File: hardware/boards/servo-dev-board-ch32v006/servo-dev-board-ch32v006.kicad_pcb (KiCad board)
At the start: 4 copper layers, 50 x 50 mm, 81 parts, among them J1 BATT JST-PH, J2 BUS JST-ZH, J3 BUS JST-ZH, J4 SERVO JST-ZH, J5 ENC JST-ZH, J6 DBG JST-ZH, Q4 AO3400A, SW1 SW_Push, U1 HT75xx-1-SOT89, U3 DRV8837DSGR-JSM, U4 CH32V006F8U6

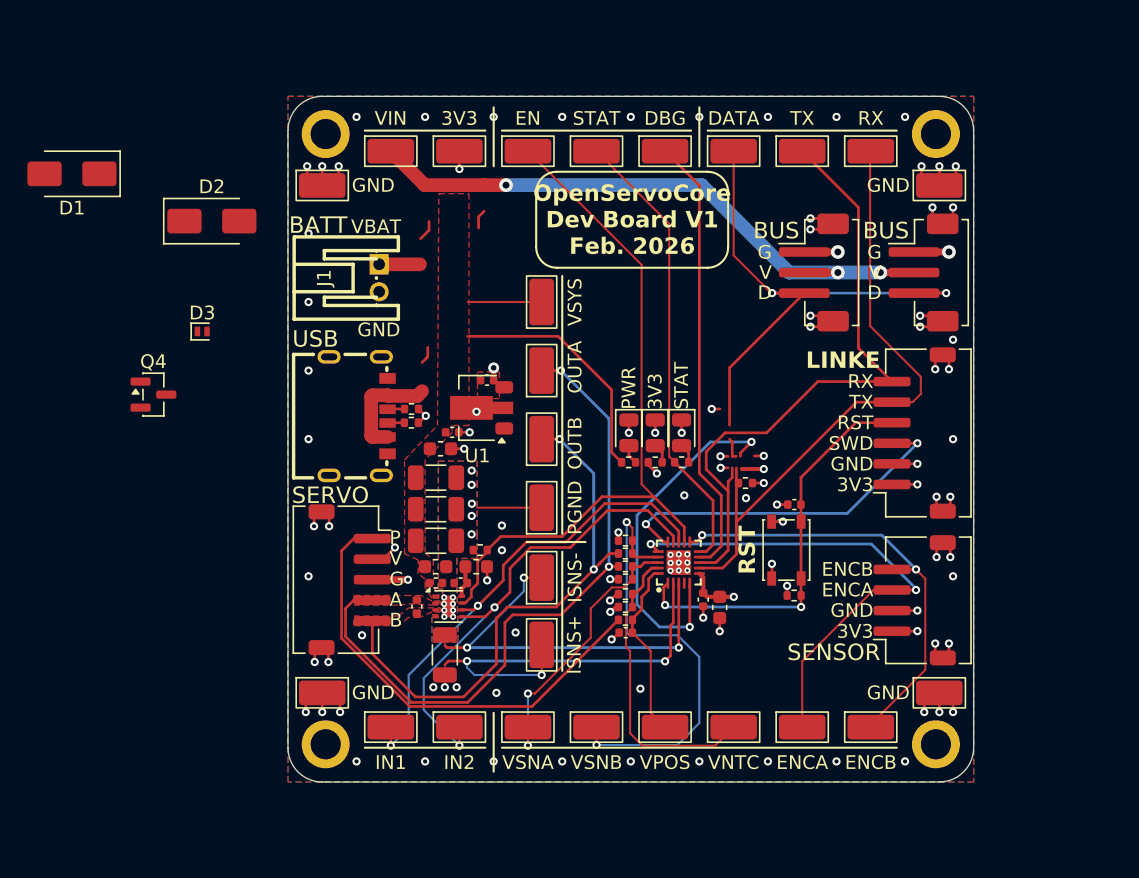
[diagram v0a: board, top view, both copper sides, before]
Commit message: completed rework
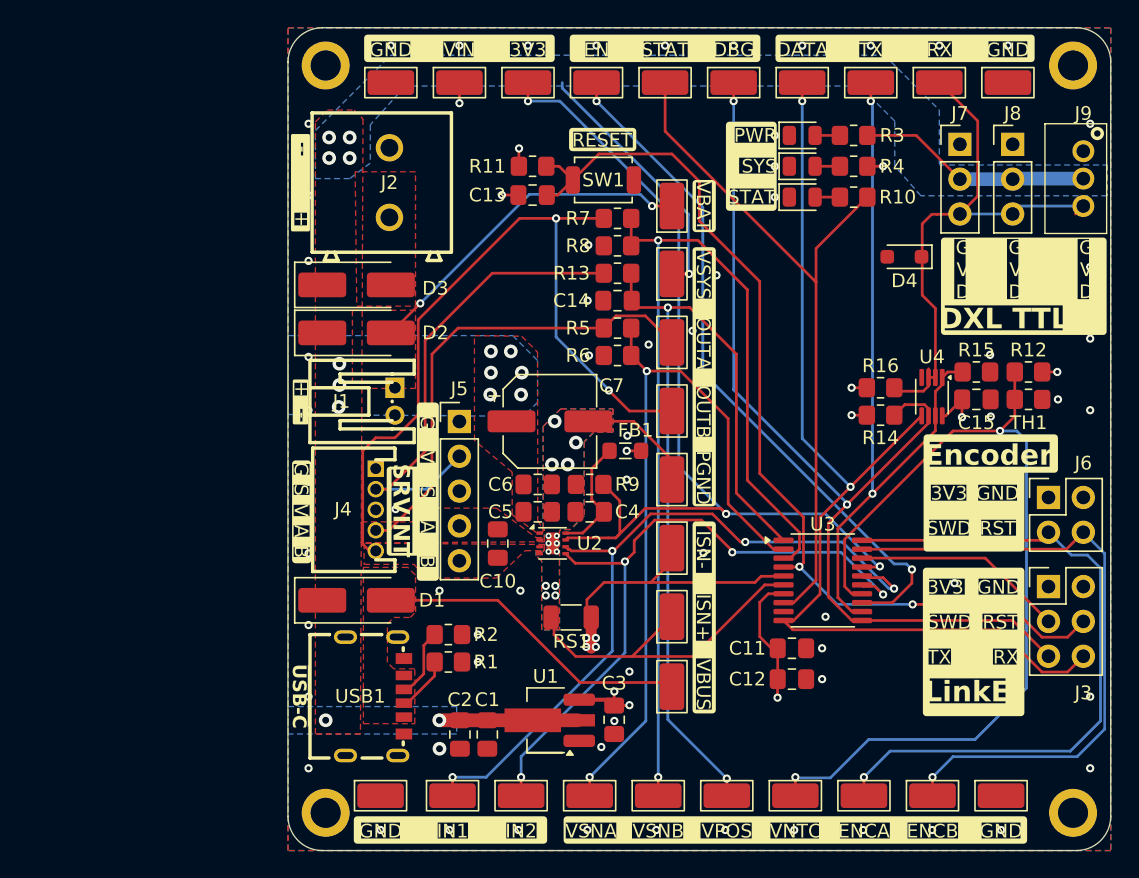
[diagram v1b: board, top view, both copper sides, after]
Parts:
- removed C8: 0.1µF, Capacitor_SMD:C_0402_1005Metric
- removed C9: 10µF, Capacitor_SMD:C_0603_1608Metric
- removed Q4: AO3400A, Package_TO_SOT_SMD:SOT-23
- removed R17: 20kΩ, Resistor_SMD:R_0402_1005Metric
- removed R18: 10kΩ, Resistor_SMD:R_0402_1005Metric
- added C4: 0.1µF, Capacitor_SMD:C_0805_2012Metric_Pad1.18x1.45mm_HandSolder, F.Cu at (152.0, 90.3)
- added D4: PESD5V0L1BA, Diode_SMD:D_SOD-323_HandSoldering, F.Cu at (174.9, 71.7)
- added J7: PIN-V, Connector_PinHeader_2.54mm:PinHeader_1x03_P2.54mm_Vertical, F.Cu at (179.0, 63.5)
- added J8: PIN-V, Connector_PinHeader_2.54mm:PinHeader_1x03_P2.54mm_Vertical, F.Cu at (182.8, 63.5)
- added J9: JST-PH-V, shared:CONN-TH_B3B-PH-K-S, F.Cu at (188.0, 66.0)
- added R1: 5.1kΩ, Resistor_SMD:R_0805_2012Metric_Pad1.20x1.40mm_HandSolder, F.Cu at (141.7, 101.2)
- added R2: 5.1kΩ, Resistor_SMD:R_0805_2012Metric_Pad1.20x1.40mm_HandSolder, F.Cu at (141.7, 99.2)
- added R3: 1.5kΩ, Resistor_SMD:R_0805_2012Metric_Pad1.20x1.40mm_HandSolder, F.Cu at (171.2, 62.9)
- added R5: 20kΩ, Resistor_SMD:R_0805_2012Metric_Pad1.20x1.40mm_HandSolder, F.Cu at (154.0, 76.9)
- added TP27: TestPoint_Probe, TestPoint:TestPoint_Keystone_5015_Micro_Mini, F.Cu at (158.0, 68.0)
- added TP28: TestPoint_Probe, TestPoint:TestPoint_Keystone_5015_Micro_Mini, F.Cu at (158.0, 103.0)
- added U2: DRV8212PDSGR, Package_SON:WSON-8-1EP_2x2mm_P0.5mm_EP0.9x1.6mm, F.Cu at (149.3, 92.6)
- C1: footprint Capacitor_SMD:C_0603_1608Metric -> Capacitor_SMD:C_0805_2012Metric_Pad1.18x1.45mm_HandSolder
- C10, C12: value 47µF -> 0.1µF; footprint Capacitor_SMD:C_1206_3216Metric -> Capacitor_SMD:C_0805_2012Metric_Pad1.18x1.45mm_HandSolder
- C11: value 47µF -> 10µF; footprint Capacitor_SMD:C_1206_3216Metric -> Capacitor_SMD:C_0805_2012Metric_Pad1.18x1.45mm_HandSolder
- C13, C15, C2, C3, C5: footprint Capacitor_SMD:C_0402_1005Metric -> Capacitor_SMD:C_0805_2012Metric_Pad1.18x1.45mm_HandSolder
- C14: value 10µF -> 0.1µF; footprint Capacitor_SMD:C_0603_1608Metric -> Capacitor_SMD:C_0805_2012Metric_Pad1.18x1.45mm_HandSolder
- C6: value 0.1µF -> 10µF; footprint Capacitor_SMD:C_0402_1005Metric -> Capacitor_SMD:C_0805_2012Metric_Pad1.18x1.45mm_HandSolder
- C7: value 0.1µF -> 100µF; footprint Capacitor_SMD:C_0402_1005Metric -> Capacitor_SMD:CP_Elec_6.3x5.4
- D1, D2: value SS34 -> SS54; footprint Diode_SMD:D_SMA -> Diode_SMD:D_SMA_Handsoldering
- D3: value ESD -> SS54; footprint Diode_SMD:D_SOD-882 -> Diode_SMD:D_SMA_Handsoldering
- FB1: footprint Inductor_SMD:L_0603_1608Metric -> Inductor_SMD:L_0805_2012Metric_Pad1.05x1.20mm_HandSolder
- J1: value BATT JST-PH -> JST-PH-H
- J2: value BUS JST-ZH -> TERM; footprint Connector_JST:JST_ZH_B3B-ZR-SM4-TF_1x03-1MP_P1.50mm_Vertical -> shared:CONN-TH_2P-P5.00_WJ500V-5.08-2P
- J3: value BUS JST-ZH -> PIN-V; footprint Connector_JST:JST_ZH_B3B-ZR-SM4-TF_1x03-1MP_P1.50mm_Vertical -> Connector_PinHeader_2.54mm:PinHeader_2x03_P2.54mm_Vertical
- J4: value SERVO JST-ZH -> JST-ZH-H; footprint Connector_JST:JST_ZH_S5B-ZR-SM4A-TF_1x05-1MP_P1.50mm_Horizontal -> shared:CONN-TH_S5B-ZR-LF-SN
- J5: value ENC JST-ZH -> PIN-V; footprint Connector_JST:JST_ZH_S4B-ZR-SM4A-TF_1x04-1MP_P1.50mm_Horizontal -> Connector_PinHeader_2.54mm:PinHeader_1x05_P2.54mm_Vertical
- J6: value DBG JST-ZH -> PIN-V; footprint Connector_JST:JST_ZH_S6B-ZR-SM4A-TF_1x06-1MP_P1.50mm_Horizontal -> Connector_PinHeader_2.54mm:PinHeader_2x02_P2.54mm_Vertical
- R10: value 5.1kΩ -> 1kΩ; footprint Resistor_SMD:R_0402_1005Metric -> Resistor_SMD:R_0805_2012Metric_Pad1.20x1.40mm_HandSolder
- R11: value 2.2kΩ -> 10kΩ; footprint Resistor_SMD:R_0402_1005Metric -> Resistor_SMD:R_0805_2012Metric_Pad1.20x1.40mm_HandSolder
- R12: value 330Ω -> 10kΩ; footprint Resistor_SMD:R_0402_1005Metric -> Resistor_SMD:R_0805_2012Metric_Pad1.20x1.40mm_HandSolder
- R13: value 1KΩ -> 4.7kΩ; footprint Resistor_SMD:R_0402_1005Metric -> Resistor_SMD:R_0805_2012Metric_Pad1.20x1.40mm_HandSolder
- R14, R16, R8: footprint Resistor_SMD:R_0402_1005Metric -> Resistor_SMD:R_0805_2012Metric_Pad1.20x1.40mm_HandSolder
- R15: value 20kΩ -> 10kΩ; footprint Resistor_SMD:R_0402_1005Metric -> Resistor_SMD:R_0805_2012Metric_Pad1.20x1.40mm_HandSolder
- R4: value 49.9Ω -> 470Ω; footprint Resistor_SMD:R_0402_1005Metric -> Resistor_SMD:R_0805_2012Metric_Pad1.20x1.40mm_HandSolder
- R6: value 4.7kΩ -> 10kΩ; footprint Resistor_SMD:R_0402_1005Metric -> Resistor_SMD:R_0805_2012Metric_Pad1.20x1.40mm_HandSolder
- R7: value 10kΩ -> 20kΩ; footprint Resistor_SMD:R_0402_1005Metric -> Resistor_SMD:R_0805_2012Metric_Pad1.20x1.40mm_HandSolder
- R9: value 5.1kΩ -> 10kΩ; footprint Resistor_SMD:R_0402_1005Metric -> Resistor_SMD:R_0805_2012Metric_Pad1.20x1.40mm_HandSolder
- RS1: value 0.1Ω 1% -> 100mΩ 1%
- SW1: footprint Button_Switch_SMD:SW_SPST_PTS810 -> Button_Switch_SMD:SW_SPST_TS-1088-xR020
- TH1: value NTC 10k -> 10kΩ 3950K; footprint Resistor_SMD:R_0402_1005Metric -> Resistor_SMD:R_0805_2012Metric_Pad1.20x1.40mm_HandSolder
- U1: value HT75xx-1-SOT89 -> HT7533-1; footprint Package_TO_SOT_SMD:SOT-89-3 -> Package_TO_SOT_SMD:SOT-89-3_Handsoldering
- U3: value DRV8837DSGR-JSM -> CH32V006F8P6; footprint Package_SON:WSON-8-1EP_2x2mm_P0.5mm_EP0.9x1.6mm -> Package_SO:TSSOP-20_4.4x6.5mm_P0.65mm
- U4: value CH32V006F8U6 -> 74LVC2G241; footprint shared:UQFN-20_L3.0-W3.0-P0.40-BL-EP1.7 -> Package_SO:VSSOP-8_2.3x2mm_P0.5mm
- USB1: value TYPE-C 6P(073) -> TYPE-C-H
- moved D1 37.4 mm to (135.0, 96.8), turned to 0 degrees
- moved R10 36.2 mm to (171.2, 67.3)
- moved J5 35.7 mm to (142.5, 83.7), turned to 0 degrees
- moved TH1 33.1 mm to (184.0, 82.1), turned to 0 degrees
- moved J2 31.6 mm to (137.4, 66.3), turned to 90 degrees
- moved SW1 30.1 mm to (153.0, 66.1), turned to 0 degrees
- moved C12 29.8 mm to (166.8, 102.5)
- moved C13 29.6 mm to (147.8, 67.2)
- moved R15 29.3 mm to (180.2, 80.1)
- moved R8 28.6 mm to (154.0, 70.9), turned to 180 degrees
- moved R12 28.0 mm to (184.0, 80.1), turned to 180 degrees
- moved C11 27.9 mm to (166.8, 100.2)
- moved U3 27.3 mm to (169.0, 95.3)
- moved C3 26.4 mm to (153.8, 105.5), turned to -90 degrees
- moved R7 26.2 mm to (154.0, 68.9), turned to 0 degrees
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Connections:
- C10 pad 1: VSYS -> /MOT_A
- C10 pad 2: PGND -> /MOT_B
- C11 pad 1: VSYS -> +3V3
- C11 pad 2: PGND -> GND
- C12 pad 1: VSYS -> +3V3
- C12 pad 2: PGND -> GND
- C13 pad 2: /nRST -> /MCU/nRST
- C14 pad 1: +3.3V -> /VPOS
- C15 pad 1: +3.3V -> +3V3
- C3 pad 1: +3.3V -> +3V3
- C5 pad 1: /VPOS -> VSYS
- C5 pad 2: GND -> PGND
- C6 pad 1: /3V3_DRV -> VSYS
- C7 pad 1: /OUTA -> VSYS
- C7 pad 2: /OUTB -> PGND
- D3 pad 1: /DATA -> VSYS
- D3 pad 2: GND -> VEXT
- FB1 pad 1: +3.3V -> +3V3
- FB1 pad 2: /3V3_DRV -> /M_DRV/+3V3_DRV
- J2 pad 1: GND -> VEXT
- J2 pad 2: VSYS -> GND
- J3 pad 1: GND -> +3V3
- J3 pad 2: VSYS -> GND
- J3 pad 3: /DATA -> /MCU/SWDIO
- J4 pad 1: /POT -> GND
- J4 pad 2: +3.3V -> /SERVO_IO/POT
- J4 pad 3: GND -> +3V3
- J4 pad 4: /OUTA -> /MOT_A
- J4 pad 5: /OUTB -> /MOT_B
- J5 pad 1: +3.3V -> GND
- J5 pad 2: GND -> /SERVO_IO/POT
- J5 pad 3: /ENCA -> +3V3
- J5 pad 4: /ENCB -> /MOT_A
- J6 pad 1: +3.3V -> +3V3
- J6 pad 3: /SWDIO -> /ENCA
- J6 pad 4: /nRST -> /ENCB
- LED1 pad 2: Net-(LED1-A) -> /POWER/LED_VSYS
- LED2 pad 2: Net-(LED2-A) -> /POWER/LED_3V3
- R10 pad 1: GND -> /STAT
- R10 pad 2: Net-(USB1-CC2) -> Net-(LED3-A)
- R11 pad 1: VSYS -> +3V3
- R11 pad 2: Net-(LED1-A) -> /MCU/nRST
- R12 pad 1: +3.3V -> +3V3
- R12 pad 2: Net-(LED2-A) -> /VNTC
- R13 pad 1: /STAT -> /VPOS
- R13 pad 2: Net-(LED3-A) -> /SERVO_IO/POT
- R14 pad 1: +3.3V -> +3V3
- R14 pad 2: /VNTC -> /RX
- R15 pad 1: /OUTA -> /TX_EN
- R15 pad 2: /VSNA -> GND
- R16 pad 1: /VSNA -> +3V3
- R16 pad 2: GND -> /DATA
- R4 pad 1: Net-(Q4-S) -> +3V3
- R4 pad 2: /UART -> /POWER/LED_3V3
- R6 pad 1: /VPOS -> /VSNA
- R6 pad 2: /POT -> GND
- R7 pad 1: /EN -> /MOT_B
- R7 pad 2: PGND -> /VSNB
- R8 pad 1: +3.3V -> /VSNB
- R8 pad 2: /nRST -> GND
- R9 pad 1: GND -> /EN
- R9 pad 2: Net-(USB1-CC1) -> PGND
- SW1 pad 1: /nRST -> /MCU/nRST
- TP12 pad 1: VBAT -> +3V3
- TP13 pad 1: +3.3V -> /EN
- TP14 pad 1: /EN -> /DBG
- TP15 pad 1: /DBG -> /STAT
- TP16 pad 1: /STAT -> /RX
- TP17 pad 1: /RX -> /TX
- TP18 pad 1: /TX -> /TX_EN
- TP22 pad 1: /OUTA -> /MOT_A
- TP23 pad 1: /OUTB -> /MOT_B
- TP25 pad 1: /ISNS+ -> /ISNS-
- TP26 pad 1: /ISNS- -> /ISNS+
- U1 pad 3: +3.3V -> +3V3
- U3 pad 1: VSYS -> /VPOS
- U3 pad 2: /OUTA -> /VSNA
- U3 pad 3: /OUTB -> /VSNB
- U3 pad 4: PGND -> /MCU/nRST
- U3 pad 5: /IN2 -> /ISNS-
- U3 pad 6: /IN1 -> /ISNS+
- U3 pad 7: /EN -> +3V3
- U3 pad 8: /3V3_DRV -> /STAT
- U3 pad 9: PGND -> GND
- U4 pad 1: /nRST -> /TX_EN
- U4 pad 2: /ISNS- -> /DATA
- U4 pad 3: /ISNS+ -> /DATA
- U4 pad 5: /UART -> /TX
- U4 pad 6: +3.3V -> /RX
- U4 pad 7: /TX -> /TX_EN
- U4 pad 8: /RX -> +3V3
- USB1 pad A5: Net-(USB1-CC1) -> /POWER/CC2
- USB1 pad B5: Net-(USB1-CC2) -> /POWER/CC1
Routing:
- net /MCU/nRST: track 0.00 -> 71.5 mm, vias 0 -> 2
- net /MOT_B: track 0.00 -> 56.2 mm, vias 0 -> 2
- net /TX_EN: track 0.00 -> 53.1 mm, vias 0 -> 2
- net /DBG: track 0.00 -> 50.8 mm, vias 0 -> 2
- net /VPOS: track 13.1 -> 63.6 mm, vias 0 -> 2
- net /OUTA: track 49.2 -> 0.00 mm, vias 2 -> 0
- net (no net): track 46.6 -> 0.00 mm
- net /VNTC: track 22.0 -> 65.5 mm, vias 0 -> 2
- net /VSNB: track 32.8 -> 74.6 mm
- net /OUTB: track 39.8 -> 0.00 mm, vias 2 -> 0
- net /SERVO_IO/POT: track 0.00 -> 35.2 mm
- net /VSNA: track 20.4 -> 55.3 mm
- net /MOT_A: track 0.00 -> 34.6 mm
- net /POT: track 33.9 -> 0.00 mm
- net GND: track 36.7 -> 3.45 mm, vias 103 -> 69
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- added copper zone on In2.Cu, net +3V3
- added copper zone on F.Cu, net /MOT_A
- added copper zone on F.Cu, net /MOT_B
- added copper zone on F.Cu, net VBAT
- added copper zone on F.Cu, net VBUS
- added copper zone on F.Cu, net VEXT
- added copper zone on B.Cu, net VSYS
- removed copper zone on F.Cu, net +3.3V
- removed copper zone on In2.Cu, net +3.3V
- removed copper zone on F.Cu, net /OUTA
- removed copper zone on F.Cu, net /OUTB
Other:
- board size 50 x 50 mm -> 60 x 60 mm
- board text added: "+"
- board text added: "-"
- board text added: "BRD: servo-dev-board-ch32v006 MCU: CH32V006F8P6 DRV: DRV8212PDSGR LDO: HT7533-1 BUF: 74LVC2G241 RS1: 0.1Ohm ~1% 250mW REV: A"
- board text added: "D3"
- board text added: "DXL TTL"
- board text added: "Encoder"
- board text added: "G V D"
- board text added: "HDR 2X2P"
- board text added: "HDR 2X3P"
- board text added: "HDR-3P"
- board text added: "ISN+"
- board text added: "ISN-"
- board text added: "JST-PH 2P"
- board text added: "JST-PH-3P"
- board text added: "JST-ZH 5P"
- board text added: "LinkE"
- board text added: "M2 Ø2.2"
- board text added: "RESET"
- board text added: "S"
- board text added: "SRVINT"
- board text added: "SYS"
- board text added: "TERM-5.08 2P"
- board text added: "USB-C PWR"
- board text added: "VBUS"
- board text removed: "BATT"
- board text removed: "BRD: servo-dev-board-ch32v006 MCU: CH32V006F8U6 DRV: DRV8837DSGR-JSM LDO: TPAP2210K-3.3TRG1 BUF: 74LVC2G125RA3-7 RS1: 0.1 OHM ~1%"
- board text removed: "BUS"
- board text removed: "D"
- board text removed: "ISNS+"
- board text removed: "ISNS-"
- board text removed: "JST-PH-2P"
- board text removed: "JST-ZH-3P"
- board text removed: "JST-ZH-4P"
- board text removed: "JST-ZH-5P"
- board text removed: "JST-ZH-6P"
- board text removed: "LINKE"
- board text removed: "P"
- board text removed: "R12"
- board text removed: "SENSOR"
- board text removed: "SERVO"
- board text removed: "USB"
